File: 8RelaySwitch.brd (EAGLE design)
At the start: 57.9 x 50.4 mm, 60 parts, among them IC1 LNK304, IC3 MC33269ST-3.3T3, K1 FRS1B, K11 FRS1B, K12 FRS1B, K13 FRS1B, K14 FRS1B, K15 FRS1B, K16 FRS1B, K2 FRS1B, T1 BC846, T2 BC846, T3 BC846, T4 BC846, T5 BC846, T6 BC846, T7 BC846, T8 BC846, X1 16 MHz

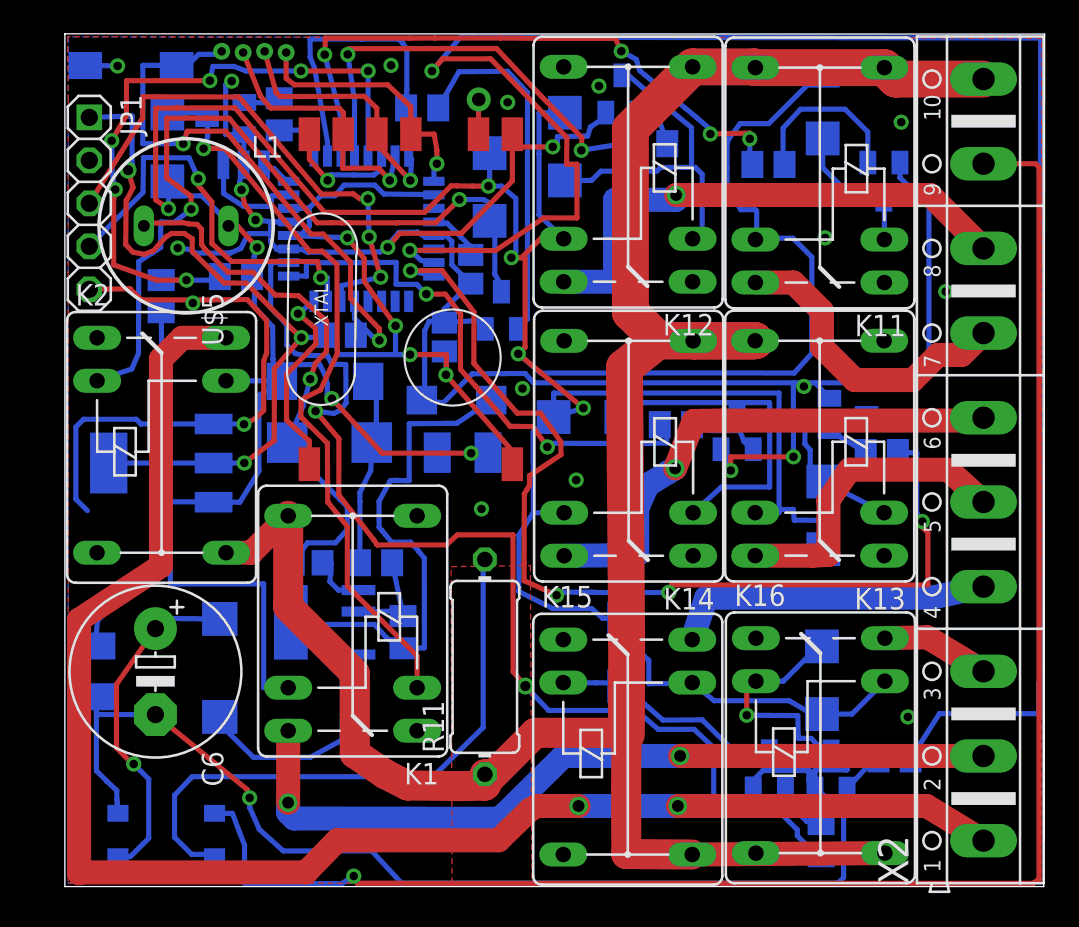
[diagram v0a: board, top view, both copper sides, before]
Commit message: aaa
aaa
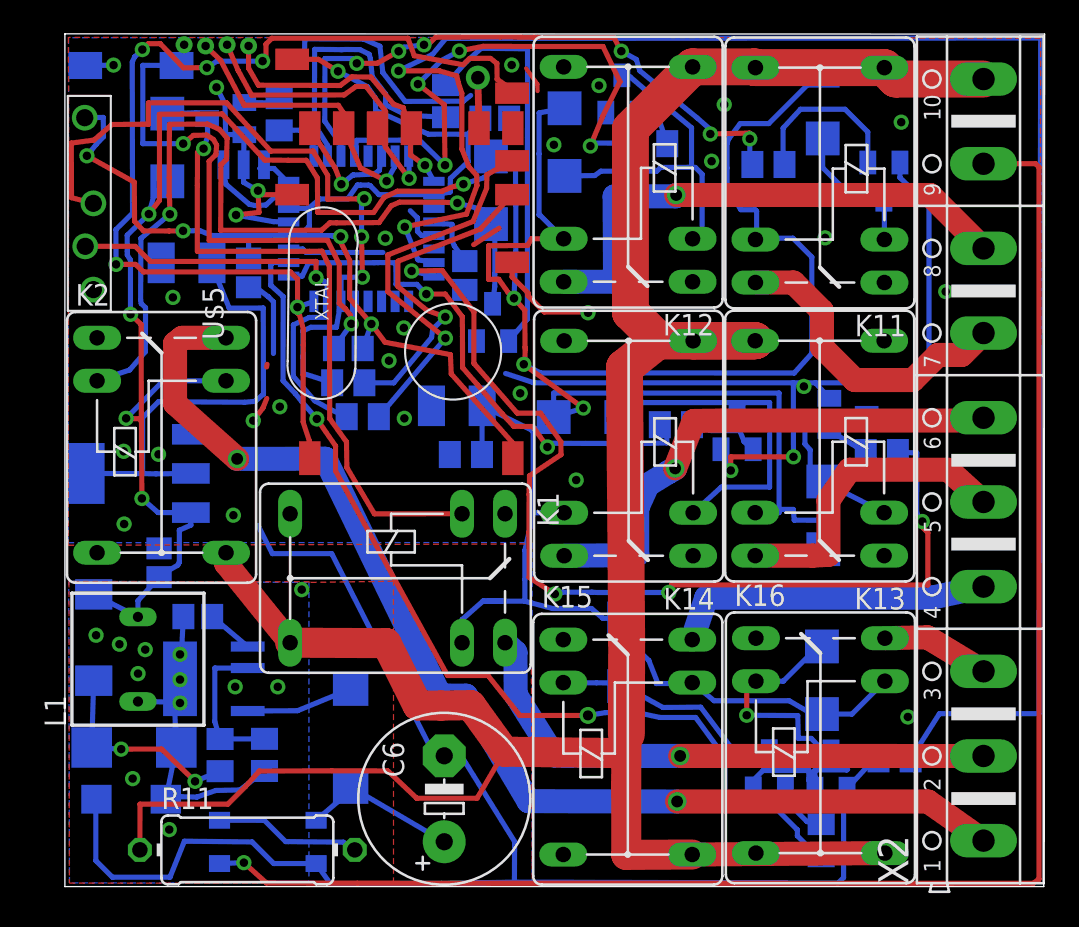
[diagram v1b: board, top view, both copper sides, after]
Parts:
- added C1, C2: 100nF, resistor:C2012
- added R16: 1 K, resistor:M2012
- added U$3: ESP03, RemoteHome:ESP03
- JP1: value (none) -> PINHD1X5SQUARE; device pinhead-2:1X05-S -> eagle-library-edeca.net-v5:PINHD1X05-SQUARE
- L1: device inductor-neosid:BS11 -> inductor-neosid:SD8
- R14: value 470 -> 1K
- R15: value 470 -> 1 K
- moved D3 30.4 mm to (3.91, 5.16)
- moved L1 25.8 mm to (4.32, 13.4), turned to 90 degrees
- moved C11 24.7 mm to (7.19, 36.9), turned to 0 degrees
- moved C8 21.4 mm to (4.09, 8.22), turned to 180 degrees
- moved D4 20.4 mm to (1.70, 14.7), turned to 90 degrees
- moved C6 18.6 mm to (22.4, 5.19), turned to 90 degrees
- moved R11 17.7 mm to (10.8, 2.17), turned to 0 degrees
- moved R14 17.2 mm to (23.7, 25.5)
- moved R12 14.6 mm to (9.17, 7.77), turned to 90 degrees
- moved R15 12.2 mm to (16.7, 29.8), turned to 0 degrees
- moved C10 12.2 mm to (10.9, 36.3), turned to 90 degrees
- moved R13 10.9 mm to (11.8, 7.78)
- moved K1 9.15 mm to (23.5, 18.2), turned to 180 degrees
- moved R10 8.77 mm to (16.9, 8.79), turned to 90 degrees
- moved IC1 7.35 mm to (8.80, 12.3)
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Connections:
- net N$10 renamed S
- new net N$10: R15.1, U$3.WIFI_TX
- new net N$12: R16.1, U$3.WIFI_RX
- net 5V1: now also C2.2
- net D0_RX: now also R15.2
- net D1_TX: now also R16.2
- net D2: now also U$3.WIFI_EN
- net D9: no longer R14.1, R15.2
- net GND: now also C1.1, C2.1, R14.1, U$3.WIFI_GND, U$3.WIFI_GPIO15; no longer R15.1
- net VCC: now also C1.2, U$3.WIFI_VDD
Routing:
- net D2: track 11.9 -> 63.0 mm, vias 1 -> 5
- net S: track 65.8 -> 19.4 mm, vias 1 -> 12
- net D9: track 39.6 -> 0.00 mm, vias 6 -> 0
- net GND: track 233.5 -> 199.5 mm, vias 23 -> 30
- net N$15: track 35.2 -> 8.66 mm
- net N$48: track 93.0 -> 68.8 mm
- net N$12: track 0.00 -> 22.7 mm, vias 0 -> 1
- net N$10: track 0.00 -> 19.6 mm, vias 0 -> 1
- net N$41: track 140.9 -> 160.0 mm
- net N$7: track 47.6 -> 33.0 mm, vias 2 -> 1
- net D0_RX: track 31.3 -> 42.3 mm
- net N$14: track 20.2 -> 9.25 mm, vias 1 -> 0
- net VCC: track 96.0 -> 104.1 mm, vias 7 -> 5
- net D4: track 64.9 -> 57.0 mm
- net N$13: track 14.0 -> 6.34 mm
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- added copper zone on layer 1, net S
- added copper zone on layer 16, net S
